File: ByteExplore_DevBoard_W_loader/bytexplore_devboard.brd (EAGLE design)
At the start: 68.6 x 53.3 mm, 91 parts, among them IC1 LM1117MPX-3.3, IC2 STM32F107RCT, IC3 CP2102, IC4 MIC5219, IC6 STM32F103C8T, J1 POWER_JACKPTH, Y1 SMD-CRYSTAL-8MHZ-20PF-20PPM(2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

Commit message: initial commit
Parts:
- C13, C22: value (none) -> 20pf
- C23, C24: value (none) -> 100nf
- R10, R20: value 220 -> 4k7
- R21: value 220 -> 100
- R23: value 220 -> 10k
- R24: value 220 -> 22
- R25: value 220 -> 222
- R26: value 220 -> 100k
- R27: value 220 -> 1k5
- R8, R9: value 220 -> 100K
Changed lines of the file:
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@@
 <attribute name="VALUE" x="17.48" y="38.83" size="1.27" layer="27" rot="R90"/>
 </element>
-<element name="C13" library="rcl" library_urn="urn:adsk.eagle:library:334" package="C0603" package3d_urn="urn:adsk.eagle:package:23616/2" value="" x="25.92" y="38.34" smashed="yes" rot="R270">
+<element name="C13" library="rcl" library_urn="urn:adsk.eagle:library:334" package="C0603" package3d_urn="urn:adsk.eagle:package:23616/2" value="20pf" x="25.92" y="38.34" smashed="yes" rot="R270">
 <attribute name="NAME" x="27.715" y="37.135" size="1.016" layer="25" font="vector" ratio="15" rot="R90"/>
 <attribute name="SPICEPREFIX" value="C" x="25.92" y="38.34" size="1.778" layer="27" rot="R270" display="off"/>
 <attribute name="VALUE" x="24.015" y="38.975" size="1.27" layer="27" rot="R270"/>
 </element>
-<element name="C22" library="rcl" library_urn="urn:adsk.eagle:library:334" package="C0603" package3d_urn="urn:adsk.eagle:package:23616/2" value="" x="25.89" y="41.55" smashed="yes" rot="R90">
+<element name="C22" library="rcl" library_urn="urn:adsk.eagle:library:334" package="C0603" package3d_urn="urn:adsk.eagle:package:23616/2" value="20pf" x="25.89" y="41.55" smashed="yes" rot="R90">
 <attribute name="NAME" x="27.865" y="40.105" size="1.016" layer="25" font="vector" ratio="15" rot="R90"/>
 <attribute name="SPICEPREFIX" value="C" x="25.89" y="41.55" size="1.778" layer="27" rot="R90" display="off"/>
 <attribute name="VALUE" x="27.795" y="40.915" size="1.27" layer="27" rot="R90"/>
 </element>
-<element name="C23" library="rcl" library_urn="urn:adsk.eagle:library:334" package="C0603" package3d_urn="urn:adsk.eagle:package:23616/2" value="" x="12.36" y="33.75" smashed="yes">
+<element name="C23" library="rcl" library_urn="urn:adsk.eagle:library:334" package="C0603" package3d_urn="urn:adsk.eagle:package:23616/2" value="100nf" x="12.36" y="33.75" smashed="yes">
 <attribute name="NAME" x="7.855" y="29.495" size="1.016" layer="25" font="vector" ratio="15"/>
 <attribute name="SPICEPREFIX" value="C" x="12.36" y="33.75" size="1.778" layer="27" display="off"/>
 <attribute name="VALUE" x="11.725" y="31.845" size="1.27" layer="27"/>
 </element>
-<element name="C24" library="rcl" library_urn="urn:adsk.eagle:library:334" package="C0603" package3d_urn="urn:adsk.eagle:package:23616/2" value="" x="20.61" y="47.19" smashed="yes" rot="R90">
+<element name="C24" library="rcl" library_urn="urn:adsk.eagle:library:334" package="C0603" package3d_urn="urn:adsk.eagle:package:23616/2" value="100nf" x="20.61" y="47.19" smashed="yes" rot="R90">
 <attribute name="NAME" x="26.315" y="49.405" size="1.016" layer="25" font="vector" ratio="15" rot="R180"/>
 <attribute name="SPICEPREFIX" value="C" x="20.61" y="47.19" size="1.778" layer="27" rot="R90" display="off"/>
 <attribute name="VALUE" x="22.515" y="46.555" size="1.27" layer="27" rot="R90"/>
 </element>
-<element name="R8" library="rcl" library_urn="urn:adsk.eagle:library:334" package="R0603" package3d_urn="urn:adsk.eagle:package:23555/2" value="220" x="18.54" y="48.03" smashed="yes" rot="R180">
+<element name="R8" library="rcl" library_urn="urn:adsk.eagle:library:334" package="R0603" package3d_urn="urn:adsk.eagle:package:23555/2" value="100K" x="18.54" y="48.03" smashed="yes" rot="R180">
 <attribute name="NAME" x="19.765" y="45.595" size="1.016" layer="25" font="vector" ratio="15" rot="R90"/>
 <attribute name="SPICEPREFIX" value="R" x="18.54" y="48.03" size="1.778" layer="27" rot="R180" display="off"/>
 <attribute name="VALUE" x="19.175" y="49.935" size="1.27" layer="27" rot="R180"/>
 </element>
-<element name="R9" library="rcl" library_urn="urn:adsk.eagle:library:334" package="R0603" package3d_urn="urn:adsk.eagle:package:23555/2" value="220" x="16.86" y="34.44" smashed="yes">
+<element name="R9" library="rcl" library_urn="urn:adsk.eagle:library:334" package="R0603" package3d_urn="urn:adsk.eagle:package:23555/2" value="100K" x="16.86" y="34.44" smashed="yes">
 <attribute name="NAME" x="16.435" y="35.315" size="1.016" layer="25" font="vector" ratio="15"/>
 <attribute name="SPICEPREFIX" value="R" x="16.86" y="34.44" size="1.778" layer="27" display="off"/>
 <attribute name="VALUE" x="16.225" y="32.535" size="1.27" layer="27"/>
 </element>
-<element name="R10" library="rcl" library_urn="urn:adsk.eagle:library:334" package="R0603" package3d_urn="urn:adsk.eagle:package:23555/2" value="220" x="12.03" y="48.63" smashed="yes">
+<element name="R10" library="rcl" library_urn="urn:adsk.eagle:library:334" package="R0603" package3d_urn="urn:adsk.eagle:package:23555/2" value="4k7" x="12.03" y="48.63" smashed="yes">
 <attribute name="NAME" x="11.395" y="46.745" size="1.016" layer="25" font="vector" ratio="15"/>
 <attribute name="SPICEPREFIX" value="R" x="12.03" y="48.63" size="1.778" layer="27" display="off"/>
 <attribute name="VALUE" x="11.395" y="46.725" size="1.27" layer="27"/>
 </element>
-<element name="R20" library="rcl" library_urn="urn:adsk.eagle:library:334" package="R0603" package3d_urn="urn:adsk.eagle:package:23555/2" value="220" x="15.27" y="48.15" smashed="yes">
+<element name="R20" library="rcl" library_urn="urn:adsk.eagle:library:334" package="R0603" package3d_urn="urn:adsk.eagle:package:23555/2" value="4k7" x="15.27" y="48.15" smashed="yes">
 <attribute name="NAME" x="23.735" y="49.405" size="1.016" layer="25" font="vector" ratio="15" rot="R180"/>
 <attribute name="SPICEPREFIX" value="R" x="15.27" y="48.15" size="1.778" layer="27" display="off"/>
 <attribute name="VALUE" x="14.635" y="46.245" size="1.27" layer="27"/>
 </element>
-<element name="R21" library="rcl" library_urn="urn:adsk.eagle:library:334" package="R0603" package3d_urn="urn:adsk.eagle:package:23555/2" value="220" x="8.7" y="48.63" smashed="yes">
+<element name="R21" library="rcl" library_urn="urn:adsk.eagle:library:334" package="R0603" package3d_urn="urn:adsk.eagle:package:23555/2" value="100" x="8.7" y="48.63" smashed="yes">
 <attribute name="NAME" x="7.015" y="46.615" size="1.016" layer="25" font="vector" ratio="15" rot="R90"/>
 <attribute name="SPICEPREFIX" value="R" x="8.7" y="48.63" size="1.778" layer="27" display="off"/>
@@
 <attribute name="VALUE" x="15.16" y="37.91" size="1.27" layer="27" rot="R180"/>
 </element>
-<element name="R23" library="rcl" library_urn="urn:adsk.eagle:library:334" package="R0603" package3d_urn="urn:adsk.eagle:package:23555/2" value="220" x="20.46" y="36.3" smashed="yes" rot="R180">
+<element name="R23" library="rcl" library_urn="urn:adsk.eagle:library:334" package="R0603" package3d_urn="urn:adsk.eagle:package:23555/2" value="10k" x="20.46" y="36.3" smashed="yes" rot="R180">
 <attribute name="NAME" x="22.165" y="35.555" size="1.016" layer="25" font="vector" ratio="15"/>
 <attribute name="SPICEPREFIX" value="R" x="20.46" y="36.3" size="1.778" layer="27" rot="R180" display="off"/>
@@
 <attribute name="VALUE" x="3.895" y="46.725" size="1.27" layer="27"/>
 </element>
-<element name="R24" library="rcl" library_urn="urn:adsk.eagle:library:334" package="R0603" package3d_urn="urn:adsk.eagle:package:23555/2" value="220" x="8.64" y="44.64" smashed="yes" rot="R180">
+<element name="R24" library="rcl" library_urn="urn:adsk.eagle:library:334" package="R0603" package3d_urn="urn:adsk.eagle:package:23555/2" value="22" x="8.64" y="44.64" smashed="yes" rot="R180">
 <attribute name="NAME" x="10.265" y="47.315" size="1.016" layer="25" font="vector" ratio="15" rot="R270"/>
 <attribute name="SPICEPREFIX" value="R" x="8.64" y="44.64" size="1.778" layer="27" rot="R180" display="off"/>
 <attribute name="VALUE" x="9.275" y="46.545" size="1.27" layer="27" rot="R180"/>
 </element>
-<element name="R25" library="rcl" library_urn="urn:adsk.eagle:library:334" package="R0603" package3d_urn="urn:adsk.eagle:package:23555/2" value="220" x="8.64" y="42.69" smashed="yes" rot="R180">
+<element name="R25" library="rcl" library_urn="urn:adsk.eagle:library:334" package="R0603" package3d_urn="urn:adsk.eagle:package:23555/2" value="222" x="8.64" y="42.69" smashed="yes" rot="R180">
 <attribute name="NAME" x="6.185" y="42.545" size="1.016" layer="25" font="vector" ratio="15" rot="R270"/>
 <attribute name="SPICEPREFIX" value="R" x="8.64" y="42.69" size="1.778" layer="27" rot="R180" display="off"/>
 <attribute name="VALUE" x="9.275" y="44.595" size="1.27" layer="27" rot="R180"/>
 </element>
-<element name="R26" library="rcl" library_urn="urn:adsk.eagle:library:334" package="R0603" package3d_urn="urn:adsk.eagle:package:23555/2" value="220" x="8.64" y="40.77" smashed="yes" rot="R180">
+<element name="R26" library="rcl" library_urn="urn:adsk.eagle:library:334" package="R0603" package3d_urn="urn:adsk.eagle:package:23555/2" value="100k" x="8.64" y="40.77" smashed="yes" rot="R180">
 <attribute name="NAME" x="10.655" y="39.925" size="1.016" layer="25" font="vector" ratio="15" rot="R180"/>
 <attribute name="SPICEPREFIX" value="R" x="8.64" y="40.77" size="1.778" layer="27" rot="R180" display="off"/>
 <attribute name="VALUE" x="9.275" y="42.675" size="1.27" layer="27" rot="R180"/>
 </element>
-<element name="R27" library="rcl" library_urn="urn:adsk.eagle:library:334" package="R0603" package3d_urn="urn:adsk.eagle:package:23555/2" value="220" x="8.67" y="46.65" smashed="yes" rot="R180">
+<element name="R27" library="rcl" library_urn="urn:adsk.eagle:library:334" package="R0603" package3d_urn="urn:adsk.eagle:package:23555/2" value="1k5" x="8.67" y="46.65" smashed="yes" rot="R180">
 <attribute name="NAME" x="6.155" y="45.545" size="1.016" layer="25" font="vector" ratio="15" rot="R270"/>
 <attribute name="SPICEPREFIX" value="R" x="8.67" y="46.65" size="1.778" layer="27" rot="R180" display="off"/>

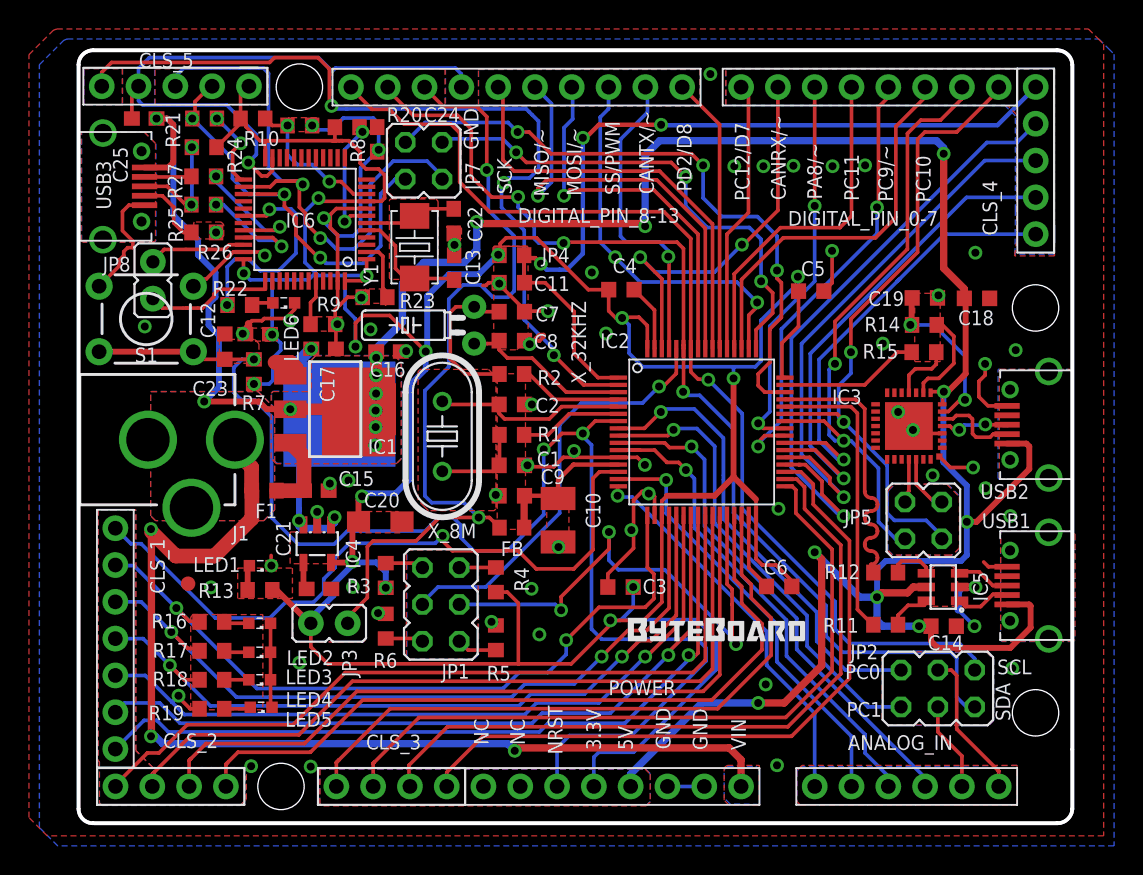
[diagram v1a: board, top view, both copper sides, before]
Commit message: initial commit add a backup file
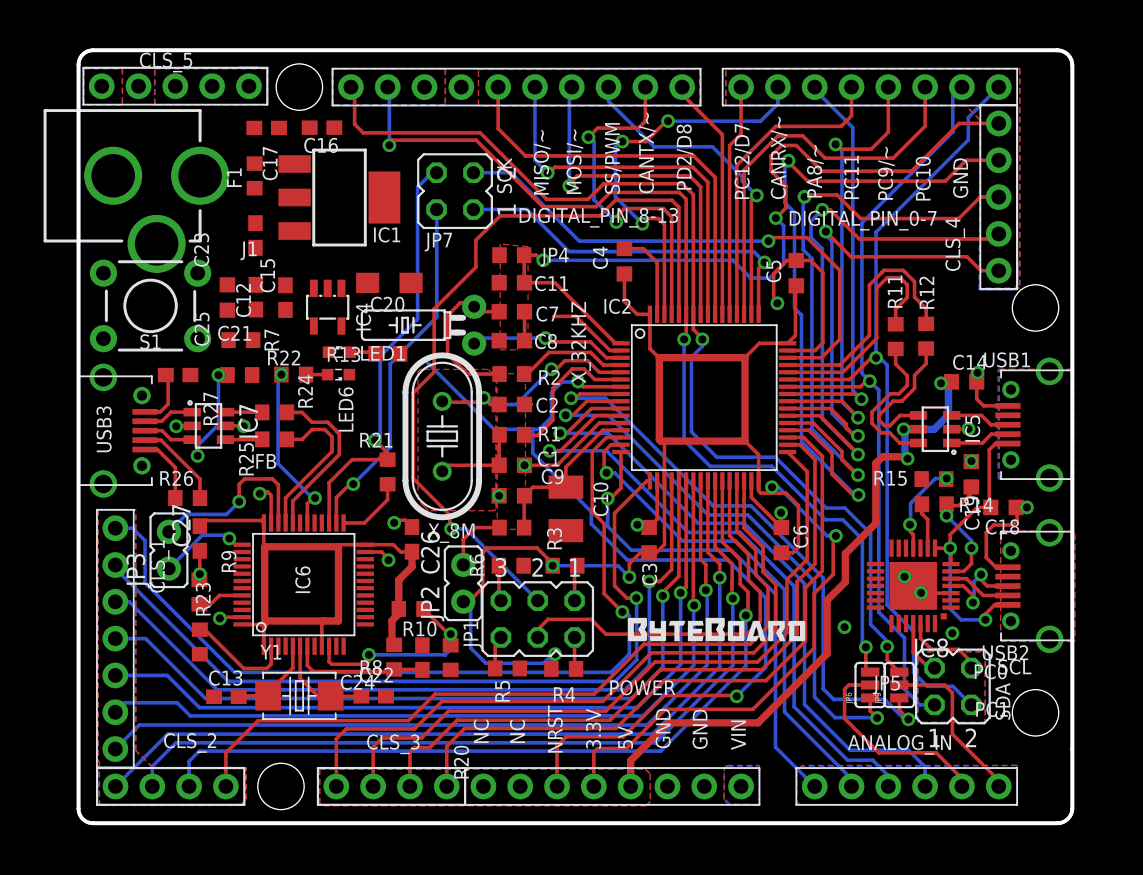
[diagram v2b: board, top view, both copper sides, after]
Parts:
- removed IC3: CP2102, silabs:MLP28
- removed JP8: (no value), jumper:JP1
- removed LED2, LED3, LED4, LED5: (no value), led:SML0603
- removed R16, R17, R18, R19: 220, rcl:R0603
- added C26, C27: (no value), rcl:C0603
- added IC7: (no value), usblc6:SOT-23-6L
- added IC8: CP2101, silabs-2:MLP28
- added JP9: JUMPER-3SMD, SparkFun:SJ_3
- JP2: device jumper:JP3Q -> jumper:JP1
- JP6: value FIDUCIAL1X2 -> JUMPER-3SMD; device SparkFun:FIDUCIAL-1X2 -> SparkFun:SJ_3
- moved JP6 47.6 mm to (54.6, 9.54), turned to 90 degrees
- moved R20 38.2 mm to (25.7, 11.4), turned to 270 degrees
- moved R8 36.7 mm to (21.8, 11.5), turned to 90 degrees
- moved C24 35.9 mm to (23.7, 11.4), turned to 270 degrees
- moved R10 35.6 mm to (22.9, 14.8)
- moved JP2 33.5 mm to (26.6, 16.6), turned to 0 degrees
- moved C13 33.5 mm to (10.2, 8.73), turned to 0 degrees
- moved C22 33.3 mm to (20.4, 8.76), turned to 180 degrees
- moved Y1 32.0 mm to (15.2, 8.79), turned to 0 degrees
- moved R21 27.5 mm to (21.3, 24.2), turned to 270 degrees
- moved R23 26.7 mm to (8.37, 12.5), turned to 270 degrees
- moved IC6 25.2 mm to (15.5, 16.5), turned to 0 degrees
- moved F1 21.7 mm to (12.2, 44.7), turned to 90 degrees
- moved R9 20.3 mm to (8.34, 16.0), turned to 90 degrees
- moved C21 20.2 mm to (14.3, 36.3), turned to 90 degrees
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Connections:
- net USB_DM renamed DW_N
- net USB_DP renamed DW_P
- removed net N$24: LED3.A, R17.2
- removed net N$25: LED4.A, R18.2
- removed net N$26: LED5.A, R19.2
- new net N$18: IC7.6, R24.2
- net +3V3: now also C26.2, C27.2, JP2.1; no longer JP3.1
- net +5V: now also IC7.5, IC8.7, IC8.8; no longer IC3.7, IC3.8
- net AN5: now also JP6.2; no longer JP2.4
- net AN6: now also JP9.2; no longer JP2.3
- net F3SWCLK: now also JP3.1; no longer JP8.1
- net F3SWDIO: now also JP3.2; no longer JP8.2
- net GND: now also C26.1, C27.1, IC7.2, IC8.3, IC8.EXP, IC8.M; no longer IC3.3, IC3.EXP, IC3.M, LED2.C, LED3.C, LED4.C, LED5.C
- net N$16: now also IC8.9; no longer IC3.9
- net N$17: now also IC8.11; no longer IC3.11
- net N$19: now also IC8.26; no longer IC3.26
- net N$20: now also IC8.25; no longer IC3.25
- net N$21: now also IC7.4, R25.2; no longer R24.2, USB3.2
- net N$23: now also IC7.1, USB3.2; no longer LED2.A, R16.2
- net N$40: now also IC7.3; no longer R25.2
- net N$5: now also IC8.6; no longer IC3.6
- net PA3: no longer R16.1
- net PA4: no longer R17.1
- net PA5: no longer R18.1
- net PA6: no longer R19.1
- net PC0: now also JP9.1; no longer JP2.5
- net PC1: now also JP6.1; no longer JP2.6
- net SCL: now also JP9.3; no longer JP2.1
- net SDA: now also JP6.3; no longer JP2.2
- net USB_N: now also IC8.5; no longer IC3.5
- net USB_P: now also IC8.4; no longer IC3.4
- net VDDA_PIN: now also JP2.2; no longer JP3.2
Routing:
- net +5V: track 249.4 -> 72.0 mm, vias 21 -> 6
- net GND: track 179.4 -> 69.6 mm, vias 64 -> 19
- net +3V3: track 243.6 -> 166.2 mm, vias 16 -> 5
- net VIN: track 72.6 -> 0.00 mm, vias 3 -> 0
- net PC13: track 59.6 -> 5.62 mm, vias 3 -> 0
- net VDDA_PIN: track 58.1 -> 4.60 mm, vias 2 -> 0
- net NRST: track 96.3 -> 64.5 mm, vias 3 -> 2
- net BOOT0: track 29.5 -> 53.6 mm
- net T_JTCK: track 39.4 -> 24.7 mm, vias 2 -> 1
- net PA0: track 47.4 -> 59.4 mm
- net RX: track 45.6 -> 56.9 mm, vias 2 -> 1
- net TX: track 43.6 -> 54.1 mm, vias 2 -> 1
- net PC2: track 35.4 -> 45.8 mm
- net PC0: track 32.0 -> 42.2 mm, vias 1 -> 2
- net PC3: track 34.3 -> 44.2 mm
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- removed copper zone on layer 1, net GND
- removed copper zone on layer 16, net GND
- removed copper zone on layer 16, net N$18
- removed copper zone on layer 1, net N$27
- removed copper zone on layer 1, net N$30
- removed copper zone on layer 1, net N$31
- removed copper zone on layer 16, net N$31
- removed copper zone on layer 1, net N$38
- removed copper zone on layer 16, net N$38
- removed copper zone on layer 1, net N$39
- removed copper zone on layer 16, net N$39
- removed copper zone on layer 1, net N$41
- removed copper zone on layer 1, net N$42
- removed copper zone on layer 1, net N$46
- removed copper zone on layer 1, net N$47
- removed copper zone on layer 1, net N$49
- removed copper zone on layer 1, net N$51
- removed copper zone on layer 1, net N$53
- removed copper zone on layer 1, net N$54
- removed copper zone on layer 1, net N$56
- removed copper zone on layer 1, net N$57
- removed copper zone on layer 16, net N$57
- removed copper zone on layer 1, net N$58
- removed copper zone on layer 1, net N$59
- removed copper zone on layer 1, net N$60
- removed copper zone on layer 1, net N$61
- removed copper zone on layer 1, net N$62
- removed copper zone on layer 1, net N$63
- removed copper zone on layer 16, net N$63
